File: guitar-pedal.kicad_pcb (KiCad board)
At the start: 2 copper layers, 63 x 117.1 mm, 50 parts, among them J1 USB_OTG, J2 AudioJack2, J3 AudioJack2, J4 Test_Headers, SW1 SW_SPDT, SW2 SW_3PDT, SW3 Boot, SW4 Reset, SW5 SW_Push_SPDT, SW6 SW_Push_SPDT, U1 Opamp_Dual, U2 MIC5504-3.3YM5, U3 ESP32-S2-SOLO, U4 PCM3002E

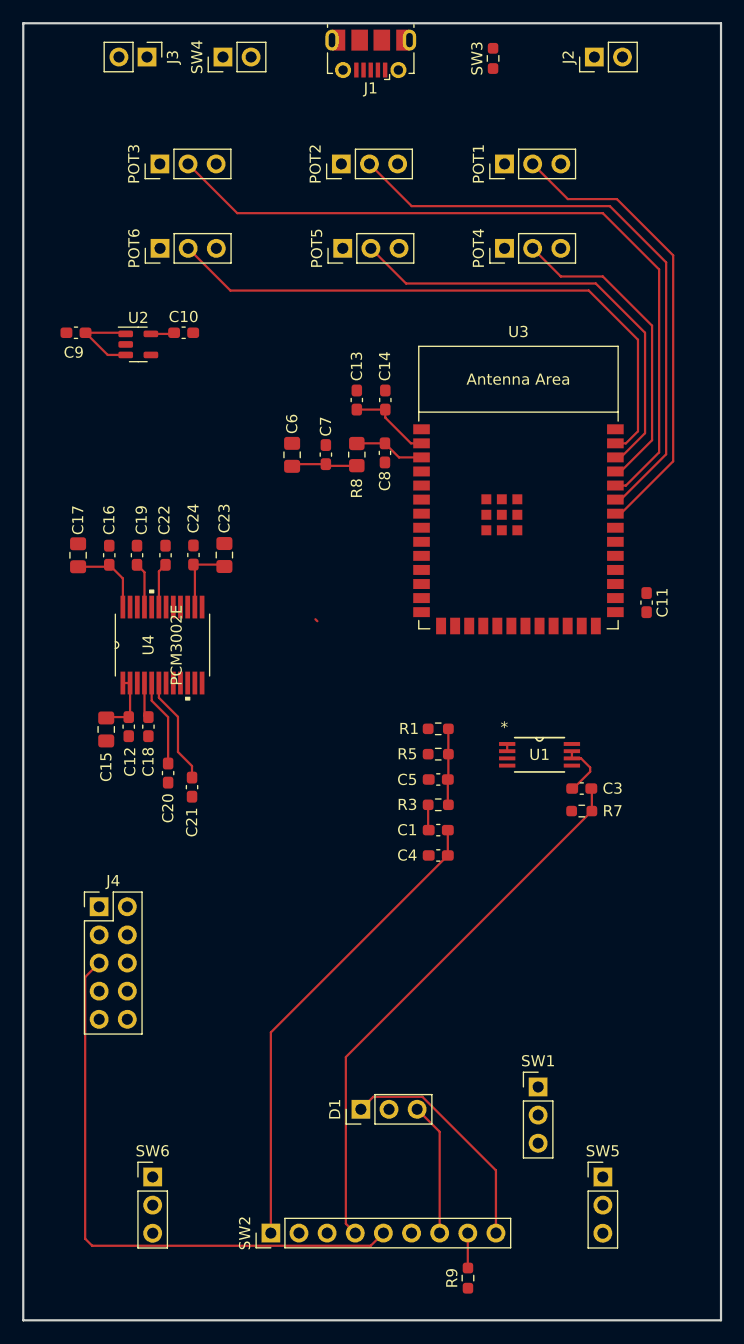
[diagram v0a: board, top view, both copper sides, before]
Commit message: layout progress!
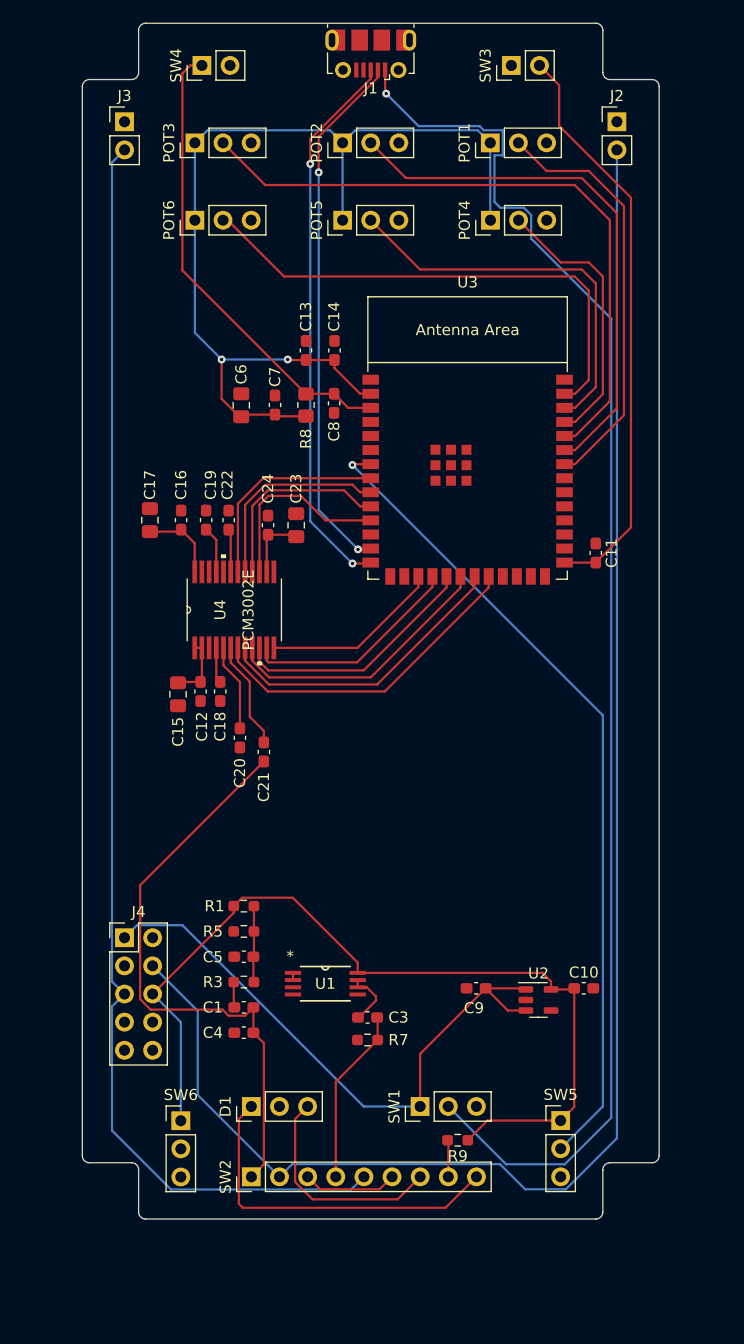
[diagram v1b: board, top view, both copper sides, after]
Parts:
- SW3: footprint Resistor_SMD:R_0603_1608Metric_Pad0.98x0.95mm_HandSolder -> Connector_PinHeader_2.54mm:PinHeader_1x02_P2.54mm_Vertical
- moved C10 69.3 mm to (155.8, 150.6)
- moved C9 69.3 mm to (146.0, 150.6)
- moved U2 69.3 mm to (151.7, 151.7)
- moved U1 28.3 mm to (132.4, 150.2)
- moved C3 28.3 mm to (136.2, 153.3)
- moved R7 28.3 mm to (136.2, 155.3)
- moved C1 23.8 mm to (125.1, 152.3)
- moved C4 23.8 mm to (125.1, 154.6)
- moved C5 23.8 mm to (125.1, 147.8)
- moved R1 23.8 mm to (125.1, 143.2)
- moved R3 23.8 mm to (125.1, 150.1)
- moved R5 23.8 mm to (125.1, 145.5)
- moved R9 12.5 mm to (144.4, 164.3), turned to 180 degrees
- moved SW1 10.8 mm to (141.0, 161.3), turned to 90 degrees
- moved D1 9.89 mm to (125.7, 161.3)
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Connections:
- U3 pad 10: /CODEC_MC -> /CODEC_ZFLG
- U3 pad 11: /CODEC_SYSCLK -> /CODEC_DATA_IN
- U3 pad 17: /CODEC_RST -> /CODEC_DATA_OUT
- U3 pad 18: /CODEC_ML -> /CODEC_BITCLK
- U3 pad 20: /CODEC_BITCLK -> /CODEC_SYSCLK
- U3 pad 21: /CODEC_DATA_OUT -> /CODEC_ML
- U3 pad 22: /CODEC_DATA_IN -> /CODEC_RST
- U3 pad 8: /CODEC_ZFLG -> /CODEC_MC
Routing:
- net +3V3: track 35.9 -> 190.3 mm, vias 0 -> 2
- net /RAW_IN: track 0.00 -> 147.0 mm
- net Net-(J1-Pad1): track 0.00 -> 128.2 mm, vias 0 -> 1
- net Net-(SW5-Pad2): track 0.00 -> 74.3 mm, vias 0 -> 1
- net /RAW_OUT: track 53.1 -> 115.4 mm
- net Net-(C11-Pad2): track 0.00 -> 52.4 mm
- net /D+: track 0.00 -> 50.1 mm, vias 0 -> 2
- net /D-: track 0.00 -> 48.1 mm, vias 0 -> 2
- net +5V: track 8.13 -> 55.2 mm
- net Net-(C8-Pad1): track 6.37 -> 42.0 mm
- net /SWITCHED_OUT: track 49.7 -> 16.0 mm
- net /CODEC_RST: track 0.00 -> 29.9 mm
- net /CODEC_ML: track 0.00 -> 27.4 mm
- net /CODEC_SYSCLK: track 0.00 -> 24.9 mm
- net /CODEC_LRCLK: track 0.00 -> 22.5 mm
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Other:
- board size 63 x 117.1 mm -> 52.1 x 107.9 mm
